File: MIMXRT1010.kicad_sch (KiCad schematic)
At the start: 26 parts, among them U1 MIMXRT1011DAE5A, Y1 32.68KHz, Y2 24 MHZ

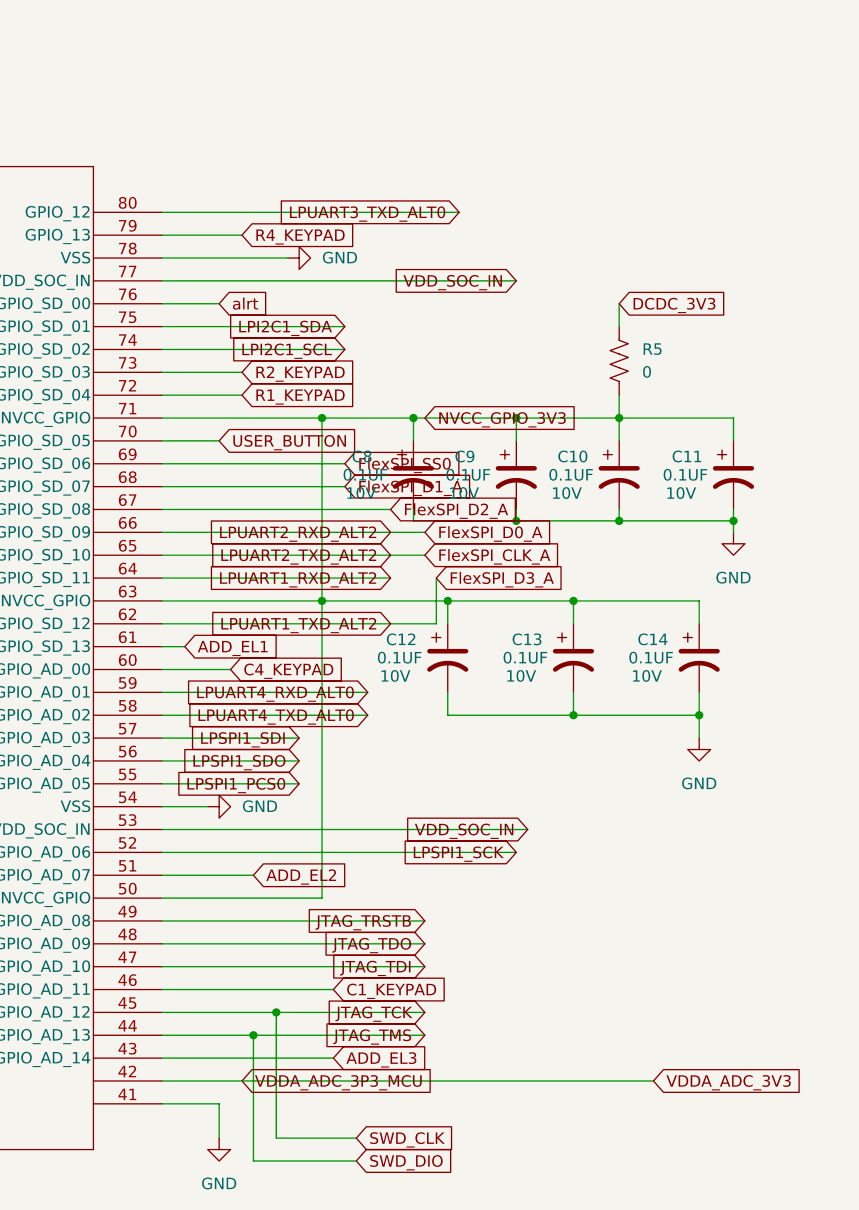
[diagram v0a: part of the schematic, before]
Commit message: add some revision
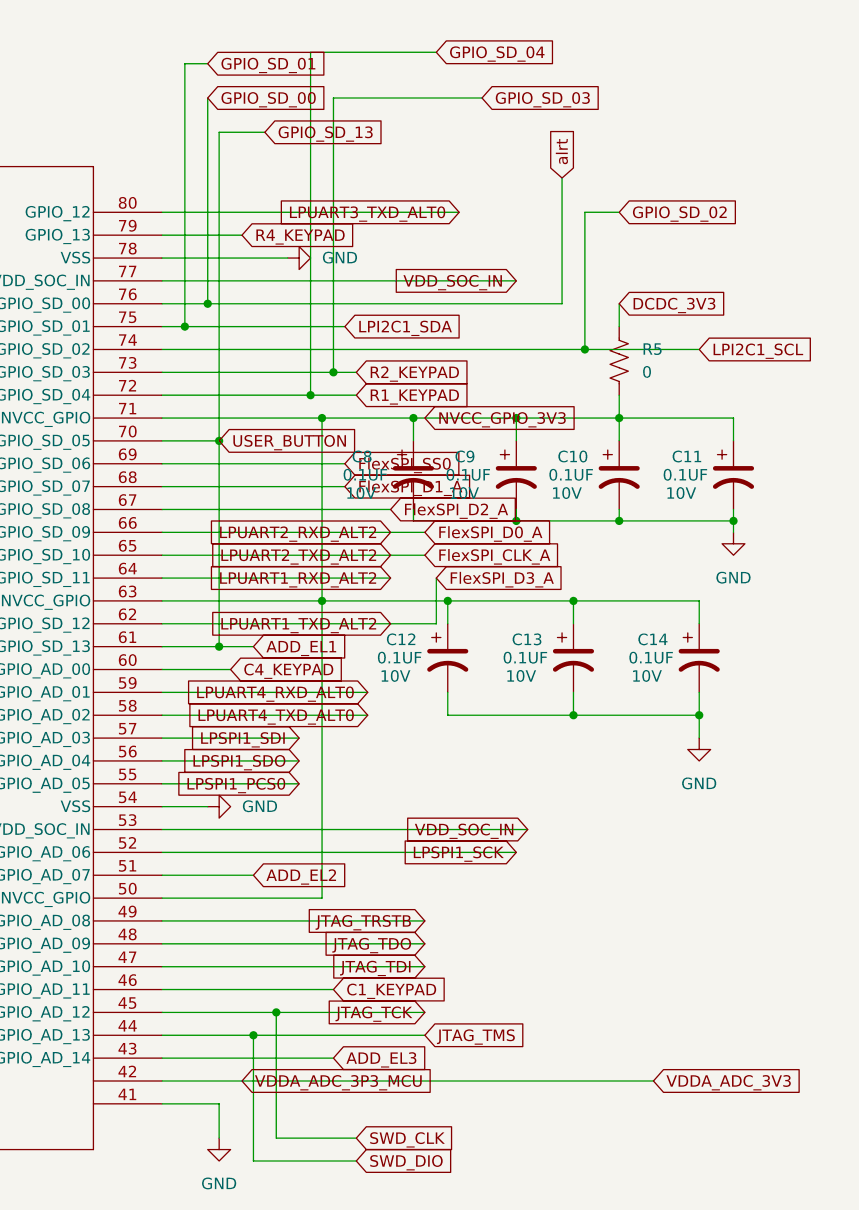
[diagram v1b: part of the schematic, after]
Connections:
- net USER_BUTTON is gone; now on net ADD_EL1: U1.70 (GPIO_SD_05)
- net LPI2C1_SCL renamed GPIO_SD_02
- net LPI2C1_SDA renamed GPIO_SD_01
- net R1_KEYPAD renamed GPIO_SD_04
- net R2_KEYPAD renamed GPIO_SD_03
- net alrt renamed GPIO_SD_00
